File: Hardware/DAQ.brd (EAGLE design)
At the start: 50 x 100 mm, 35 parts, among them IC2 FT232RL, U1 DAC8564IAPW, U2 AD7606BSTZ, X1 PN61729-S

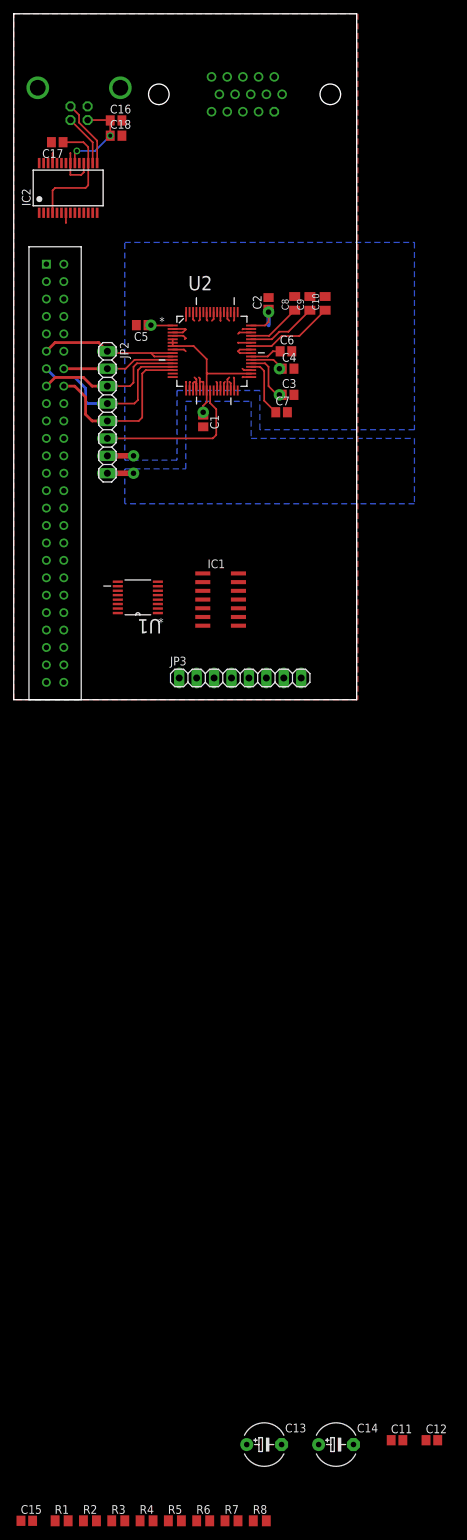
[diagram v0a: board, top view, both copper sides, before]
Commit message: finished board layout
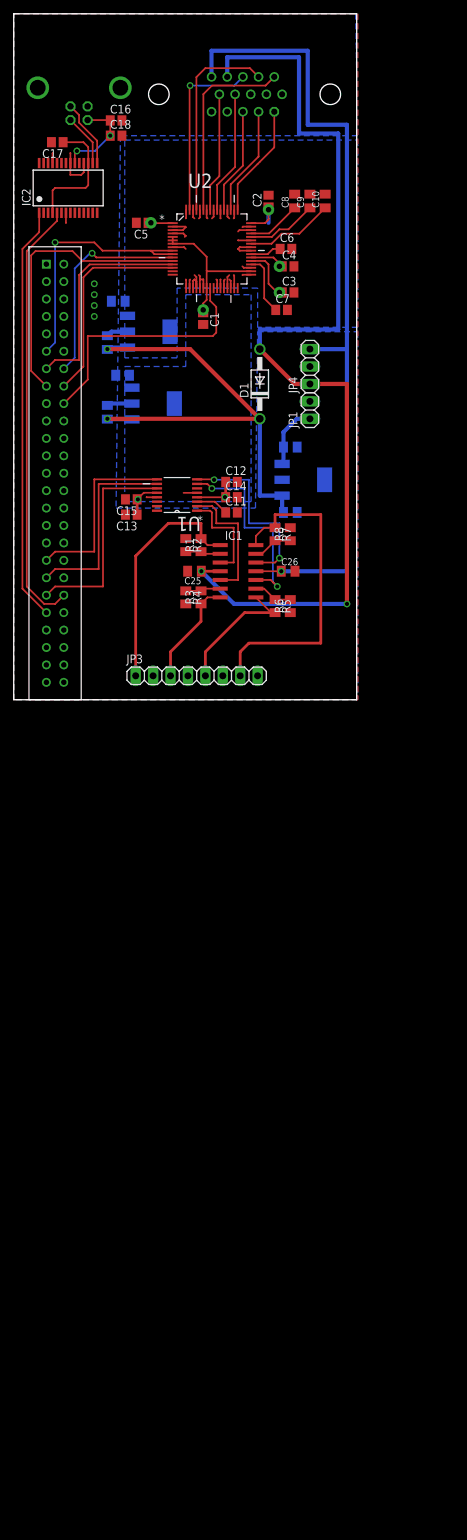
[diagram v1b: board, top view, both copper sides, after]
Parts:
- removed JP2: (no value), pinhead:1X08
- added C19, C20, C21, C22, C23, C24, C25, C26: (no value), resistor:C0805K
- added D1: 1N4004, diode:DO41-10
- added IC3, IC4, IC5: MCP1703DB, linear:SOT223
- added JP1: (no value), pinhead:1X02
- added JP4: (no value), pinhead:1X03
- C13, C14: device resistor:E5-6 -> resistor:C0805
- moved C15 149.7 mm to (17.1, 29.2), turned to 180 degrees
- moved R7 144.0 mm to (38.1, 24.1), turned to 270 degrees
- moved R8 143.9 mm to (40.3, 24.1), turned to 90 degrees
- moved R1 143.7 mm to (27.3, 22.5), turned to 90 degrees
- moved R2 142.9 mm to (25.1, 22.5), turned to 270 degrees
- moved C12 142.7 mm to (31.8, 31.8)
- moved C14 139.0 mm to (31.8, 29.5)
- moved C11 137.4 mm to (31.8, 27.3)
- moved C13 136.9 mm to (17.1, 27.0), turned to 180 degrees
- moved R3 135.2 mm to (27.3, 14.9), turned to 90 degrees
- moved R4 134.7 mm to (25.1, 14.9), turned to 270 degrees
- moved R5 134.1 mm to (38.1, 13.7), turned to 270 degrees
- moved R6 134.0 mm to (40.3, 13.7), turned to 90 degrees
- moved U1 16.0 mm to (23.8, 29.8)
- moved C7 14.9 mm to (39.1, 56.8)
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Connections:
- removed net V+: IC1.4
- removed net V-: IC1.11
- new net N$12: C21.1, IC5.3, JP1.1
- new net N$29: C22.1, C23.1, C24.1, D1.C, IC3.1, IC4.1, IC5.1
- net +15V: now also C25.1, D1.A, IC1.4, JP4.1
- net +3V3: now also C13.1, C14.1, C20.1, IC3.3; no longer C13.+, C14.+, JP2.8
- net +5V: now also C19.1, IC4.3; no longer JP2.7
- net -15V: now also C26.1, IC1.11, JP4.3
- net BUSY: no longer JP2.5
- net CONVST: no longer JP2.1
- net CS: no longer JP2.4
- net GND: now also C13.2, C14.2, C19.2, C20.2, C21.2, C22.2, C23.2, C24.2, C25.2, C26.2, IC3.2, IC4.2, IC5.2, JP1.2, JP4.2; no longer C13.-, C14.-
- net RESET: no longer JP2.2
- net SPI1_MISO: no longer JP2.6
- net SPI1_SCLK: no longer JP2.3
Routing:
- net +15V: track 0.00 -> 145.9 mm, vias 0 -> 2
- net -15V: track 0.00 -> 118.2 mm, vias 0 -> 1
- net N$29: track 0.00 -> 72.5 mm, vias 0 -> 2
- net USART3_TX: track 0.00 -> 63.3 mm
- net USART3_RX: track 0.00 -> 60.7 mm
- net N$25: track 0.00 -> 47.7 mm
- net N$19: track 0.00 -> 34.4 mm
- net SPI2_MOSI: track 0.00 -> 31.0 mm
- net Q4_BUF: track 0.00 -> 29.5 mm
- net N$16: track 0.00 -> 29.4 mm, vias 0 -> 2
- net SPI2_SCLK: track 0.00 -> 29.1 mm
- net Q3_BUF: track 0.00 -> 28.2 mm
- net ~SYNC: track 0.00 -> 27.2 mm
- net N$17: track 0.00 -> 27.2 mm, vias 0 -> 2
- net Q2-Q3_BUF: track 0.00 -> 26.3 mm, vias 0 -> 1
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- added copper zone on layer 16, net GND
